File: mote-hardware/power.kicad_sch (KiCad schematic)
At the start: 8 parts, among them J1 USB_C_Receptacle_USB2.0_14P, U10 TPD2E2U06DCK, U2 NCP1117-3.3_SOT223, U3 USBLC6-2SC6

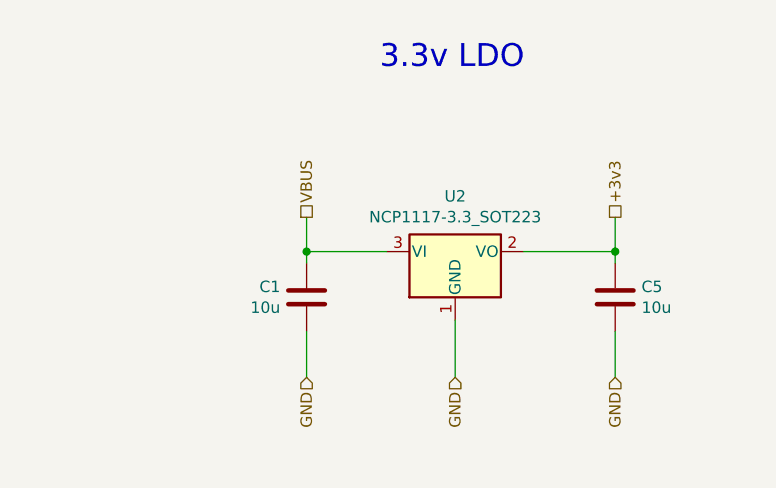
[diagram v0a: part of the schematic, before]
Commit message: Small tweaks and fixes to the schematic (#68)
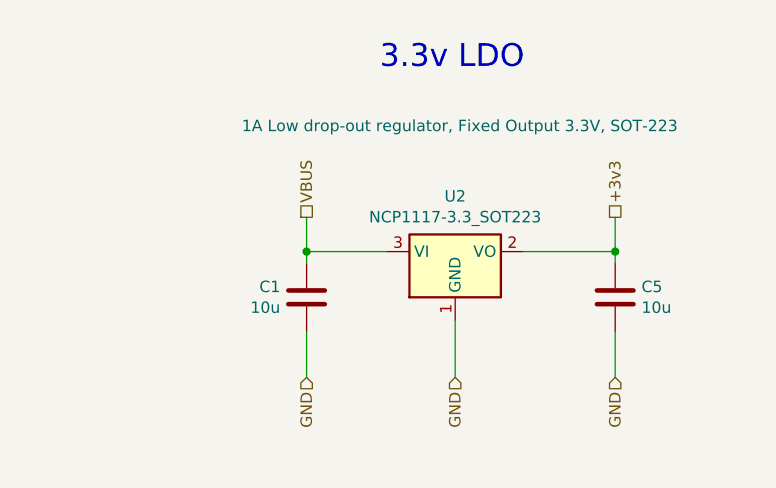
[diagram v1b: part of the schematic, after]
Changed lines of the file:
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@@
 	(title_block
 		(title "Mote")
-		(date "2026-05-25")
+		(date "2026-06-07")
 		(rev "V0.2.0")
 		(company "github.com/empriselab/mote")
@@
 			)
 		)
-		(property "Description" ""
-			(at 233.68 99.06 0)
+		(property "Description" "1A Low drop-out regulator, Fixed Output 3.3V, SOT-223"
+			(at 234.188 85.09 0)
 			(effects
 				(font
